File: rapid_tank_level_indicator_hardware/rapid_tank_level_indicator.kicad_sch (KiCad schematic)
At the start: 83 parts, among them J1 Conn_01x04_Pin, J17 TC2050, J2 Conn_02x04_Top_Bottom, J3 Conn_02x04_Top_Bottom, SW1 KMR721NGLFS, SW2 KMR721NGLFS, U1 L7805, U10 MCP9700Ax-ETT, U11 TPD4E1U06, U12 MCP9700Ax-ETT, U13 MCP9700Ax-ETT, U14 MCP9700Ax-ETT, U15 MCP9700Ax-ETT, U16 MCP2562-E-SN, U2 L7805, U3 STM32F105RCTx, U4 MCP9700Ax-ETT, U5 AZ1117-3.3, U6 MCP9700Ax-ETT, U7 MCP9700Ax-ETT, U8 MCP9700Ax-ETT, U9 MCP9700Ax-ETT, Y1 8MHz 12pF

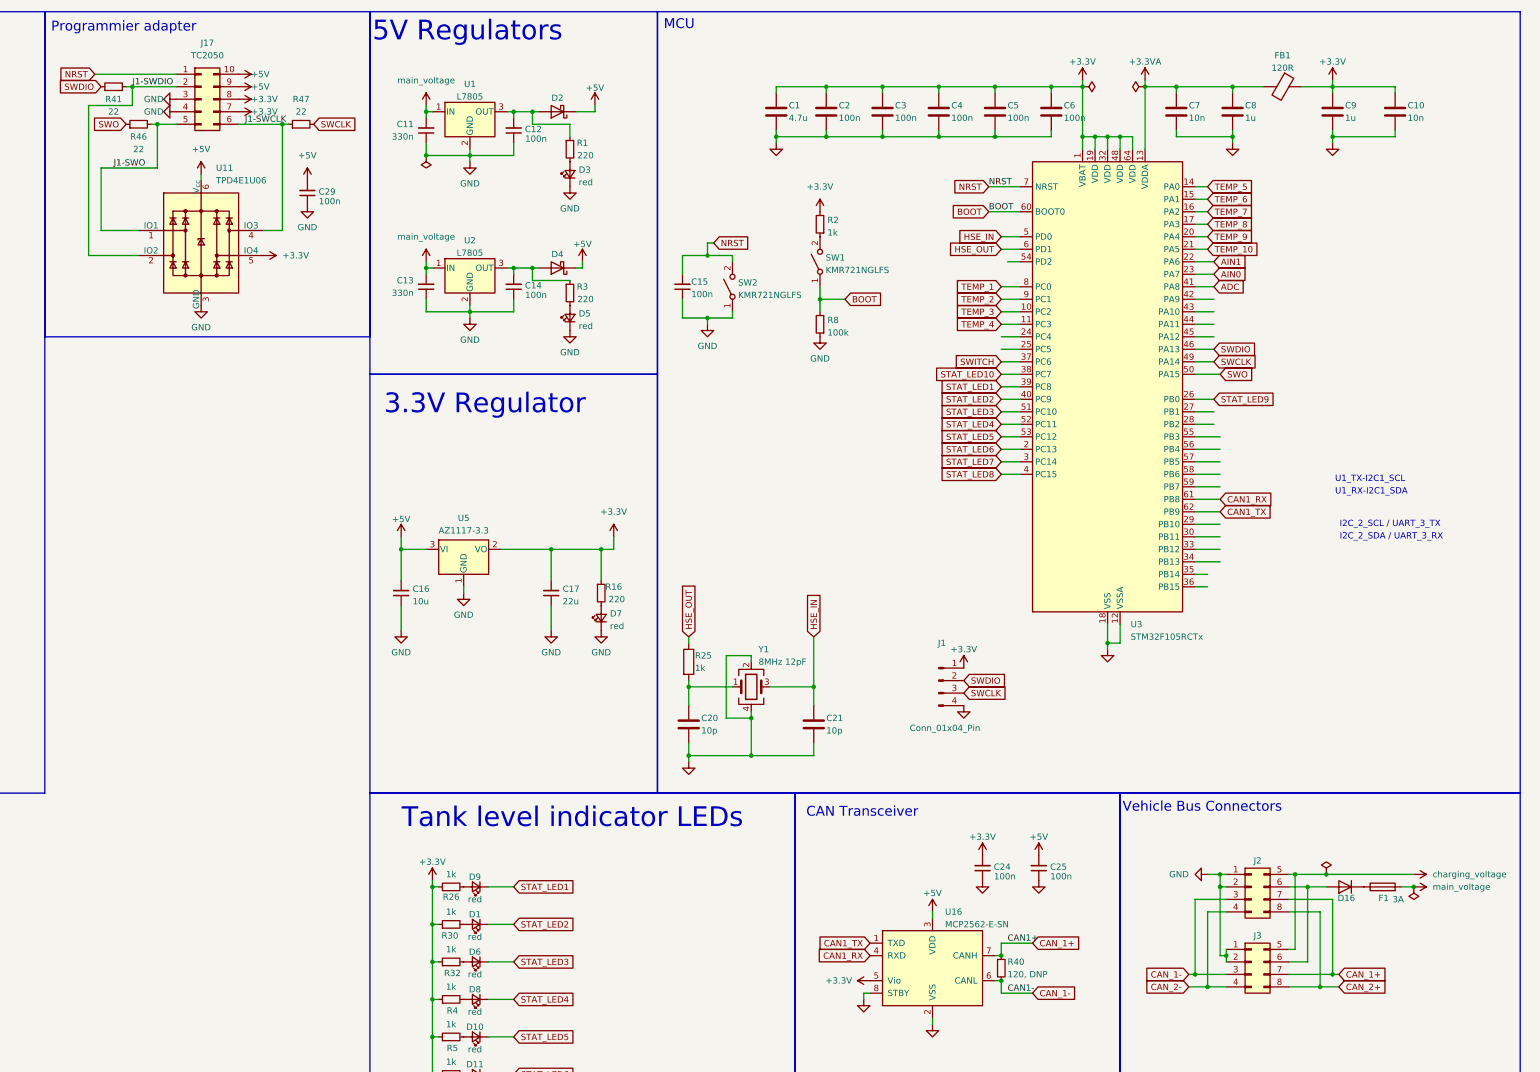
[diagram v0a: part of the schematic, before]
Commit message: finish design
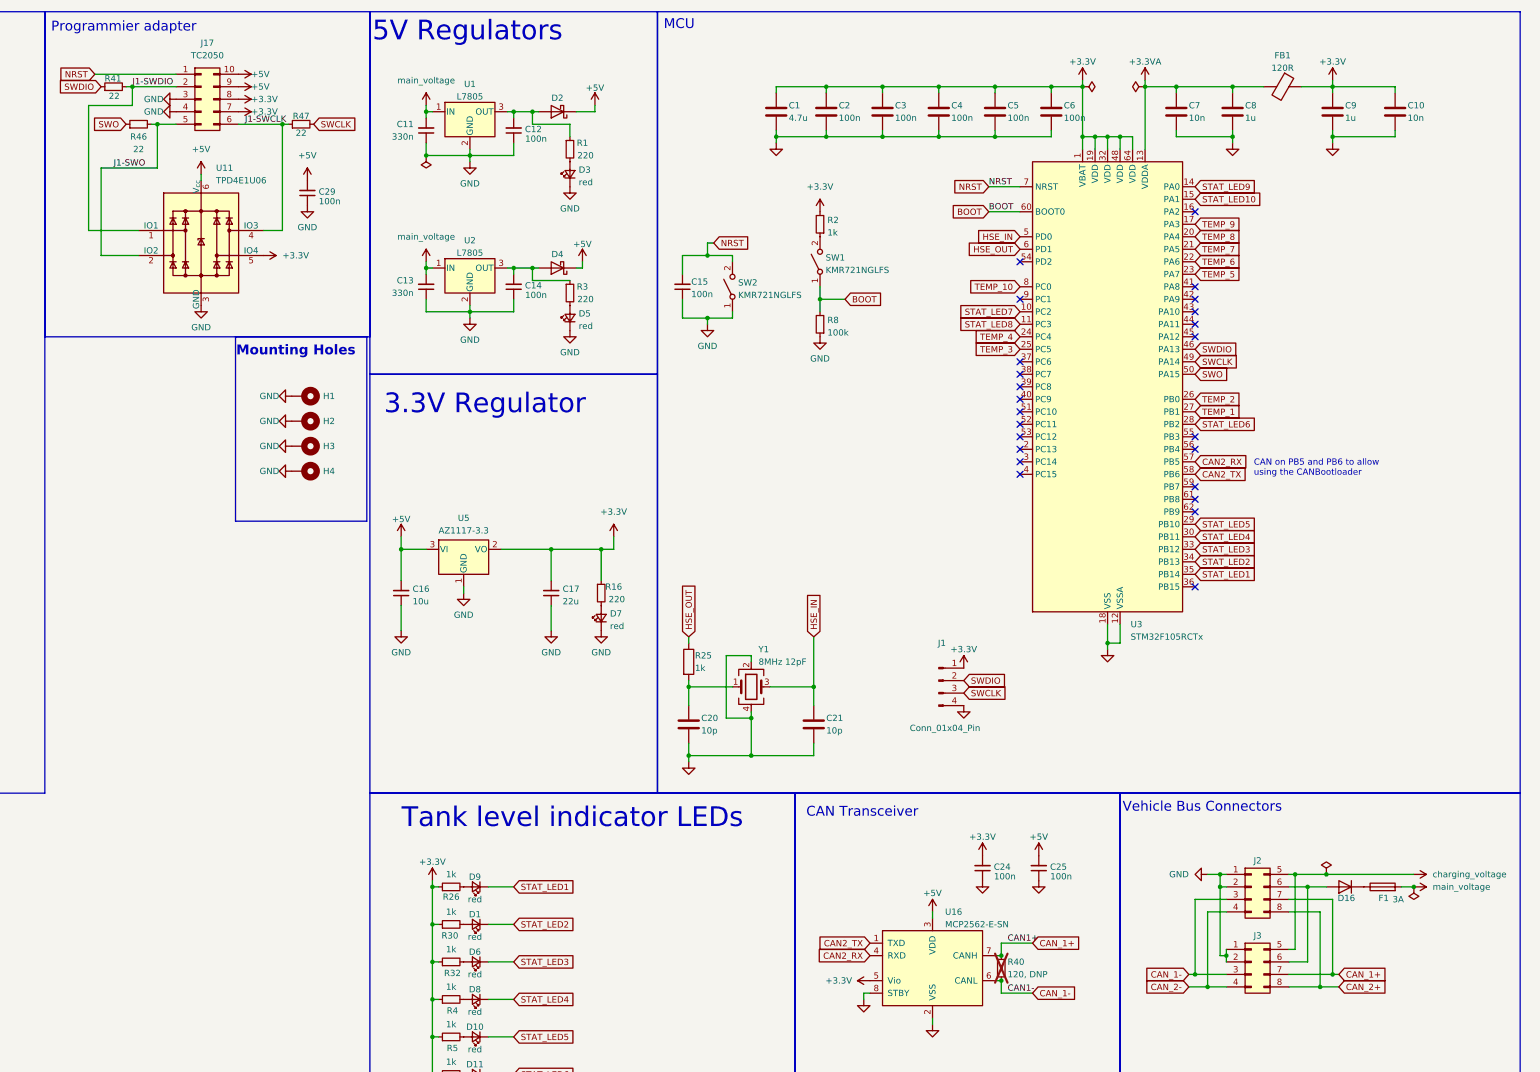
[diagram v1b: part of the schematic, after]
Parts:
- added H1, H2, H3, H4: MountingHole_Pad, MountingHole:MountingHole_3.2mm_M3_Pad_Via, symbol Mechanical:MountingHole_Pad
- R40: now not fitted
- U10, U12, U13, U14, U15, U4, U6, U7, U8, U9: LCSC (none) -> C127949
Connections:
- net AIN0 is gone; now on net TEMP_5: U3.23 (PA7)
- net AIN1 is gone; now on net TEMP_6: U3.22 (PA6)
- net GND: now also H1.1, H2.1, H3.1, H4.1
- net J1-SWDIO: now also U11.1 (IO1); no longer U11.2 (IO2)
- net J1-SWO: now also U11.2 (IO2); no longer U11.1 (IO1)
- net STAT_LED1: now also U3.35 (PB14); no longer U3.39 (PC8)
- net STAT_LED10: now also U3.15 (PA1); no longer U3.38 (PC7)
- net STAT_LED2: now also U3.34 (PB13); no longer U3.40 (PC9)
- net STAT_LED3: now also U3.33 (PB12); no longer U3.51 (PC10)
- net STAT_LED4: now also U3.30 (PB11); no longer U3.52 (PC11)
- net STAT_LED5: now also U3.29 (PB10); no longer U3.53 (PC12)
- net STAT_LED6: now also U3.28 (PB2); no longer U3.2 (PC13)
- net STAT_LED7: now also U3.10 (PC2); no longer U3.3 (PC14)
- net STAT_LED8: now also U3.11 (PC3); no longer U3.4 (PC15)
- net STAT_LED9: now also U3.14 (PA0); no longer U3.26 (PB0)
- net TEMP_1: now also U3.27 (PB1); no longer U3.8 (PC0)
- net TEMP_10: now also U3.8 (PC0); no longer U3.21 (PA5)
- net TEMP_2: now also U3.26 (PB0); no longer U3.9 (PC1)
- net TEMP_3: now also U3.25 (PC5); no longer U3.10 (PC2)
- net TEMP_4: now also U3.24 (PC4); no longer U3.11 (PC3)
- net TEMP_5: no longer U3.14 (PA0)
- net TEMP_6: no longer U3.15 (PA1)
- net TEMP_7: now also U3.21 (PA5); no longer U3.16 (PA2)
- net TEMP_8: now also U3.20 (PA4); no longer U3.17 (PA3)
- net TEMP_9: now also U3.17 (PA3); no longer U3.20 (PA4)
- net CAN2_RX: now reaches U3.57 (PB5)
- net CAN2_RX: now also U16.4 (RXD)
- net CAN2_TX: now reaches U3.58 (PB6)
- net CAN2_TX: now also U16.1 (TXD)
- net ADC: no longer names the net of U3.41 (PA8)
- net CAN1_RX: no longer names the net of U3.61 (PB8)
- net CAN1_RX: no longer U16.4 (RXD)
- net CAN1_TX: no longer names the net of U3.62 (PB9)
- net CAN1_TX: no longer U16.1 (TXD)
- net SWITCH: no longer names the net of U3.37 (PC6)
- no-connect marks 0 -> 24
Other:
- note added: "CAN on PB5 and PB6 to allow using the CANBootloader"
- note added: "Mounting Holes"
- note removed: "I2C_2_SCL / UART_3_TX"
- note removed: "I2C_2_SDA / UART_3_RX"
- note removed: "U1_RX-I2C1_SDA"
- note removed: "U1_TX-I2C1_SCL"
